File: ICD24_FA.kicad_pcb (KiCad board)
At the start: 2 copper layers, 201.5 x 218 mm, 446 parts, among them J1 Conn_01x02, Q342 2N3904, Q343 2N3904, Q344 2N3904, Q345 2N3904, Q346 2N3904, Q347 2N3904, Q348 2N3904, Q349 2N3904, Q350 2N3904, Q351 2N3904, Q352 2N3904, Q353 2N3904, Q354 2N3904, Q355 2N3904, Q356 2N3904, Q357 2N3904, Q358 2N3904, Q359 2N3904, Q360 2N3904, Q361 2N3904, Q362 2N3904, Q363 2N3904, Q364 2N3904, Q365 2N3904, Q366 2N3904, Q367 2N3904, Q368 2N3904, Q369 2N3904, Q370 2N3904, Q371 2N3904, Q372 2N3904, Q373 2N3904, Q374 2N3904, Q375 2N3904, Q376 2N3904, Q377 2N3904, Q378 2N3904, Q379 2N3904, Q380 2N3904, Q381 2N3904, Q382 2N3904, Q383 2N3904, Q384 2N3904, Q385 2N3904, Q386 2N3904, Q387 2N3904, Q388 2N3904, Q389 2N3904, Q390 2N3904, Q391 2N3904, Q392 2N3904, Q393 2N3904, Q394 2N3904, Q395 2N3904, Q396 2N3904, Q397 2N3904, Q398 2N3904, Q399 2N3904, Q400 2N3904, Q401 2N3904, Q402 2N3904, Q403 2N3904, Q404 2N3904, Q405 2N3904, Q406 2N3904, Q407 2N3904, Q408 2N3904, Q409 2N3904, Q410 2N3904, Q411 2N3904, Q412 2N3904, Q413 2N3904, Q414 2N3904, Q415 2N3904, Q416 2N3904, Q417 2N3904, Q418 2N3904, Q419 2N3904, Q420 2N3904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

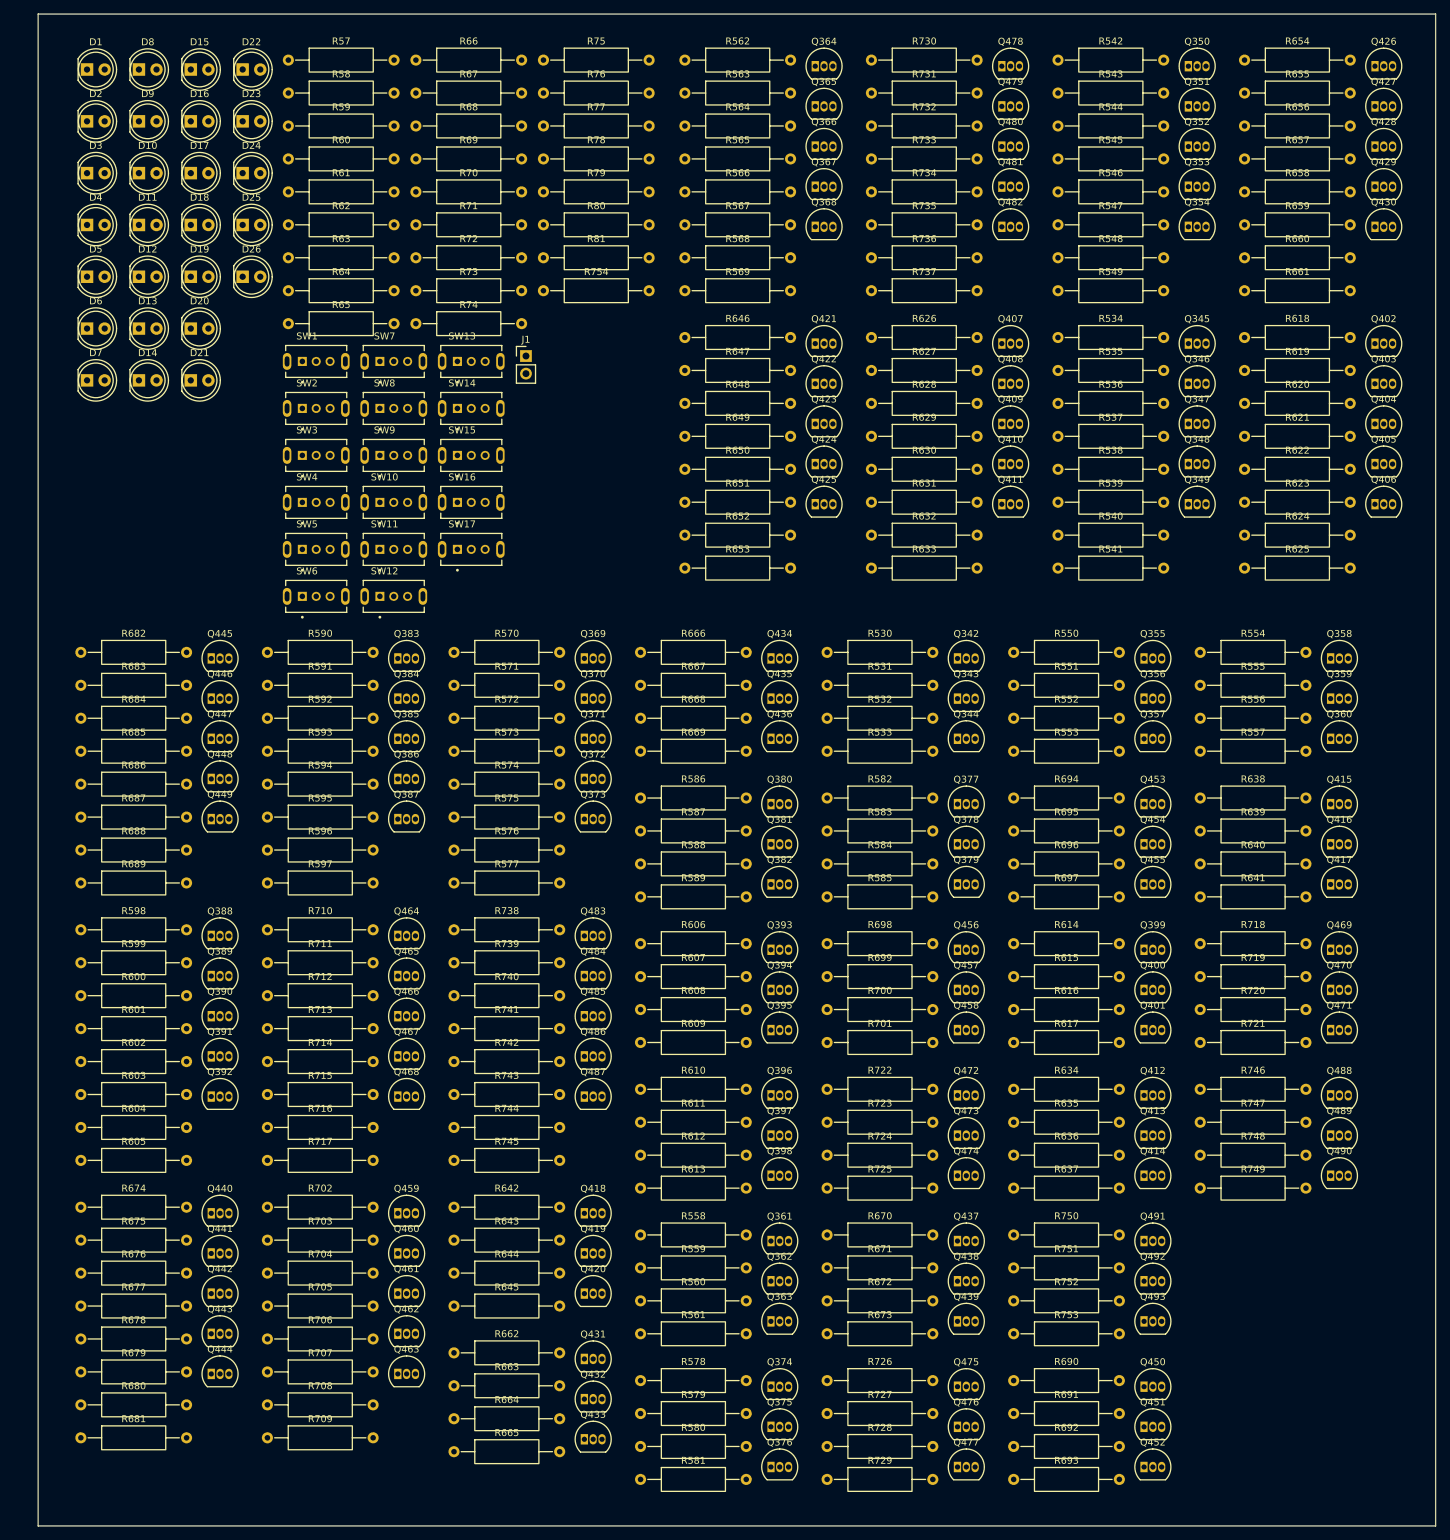
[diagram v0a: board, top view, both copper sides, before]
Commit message: FA 2-bit
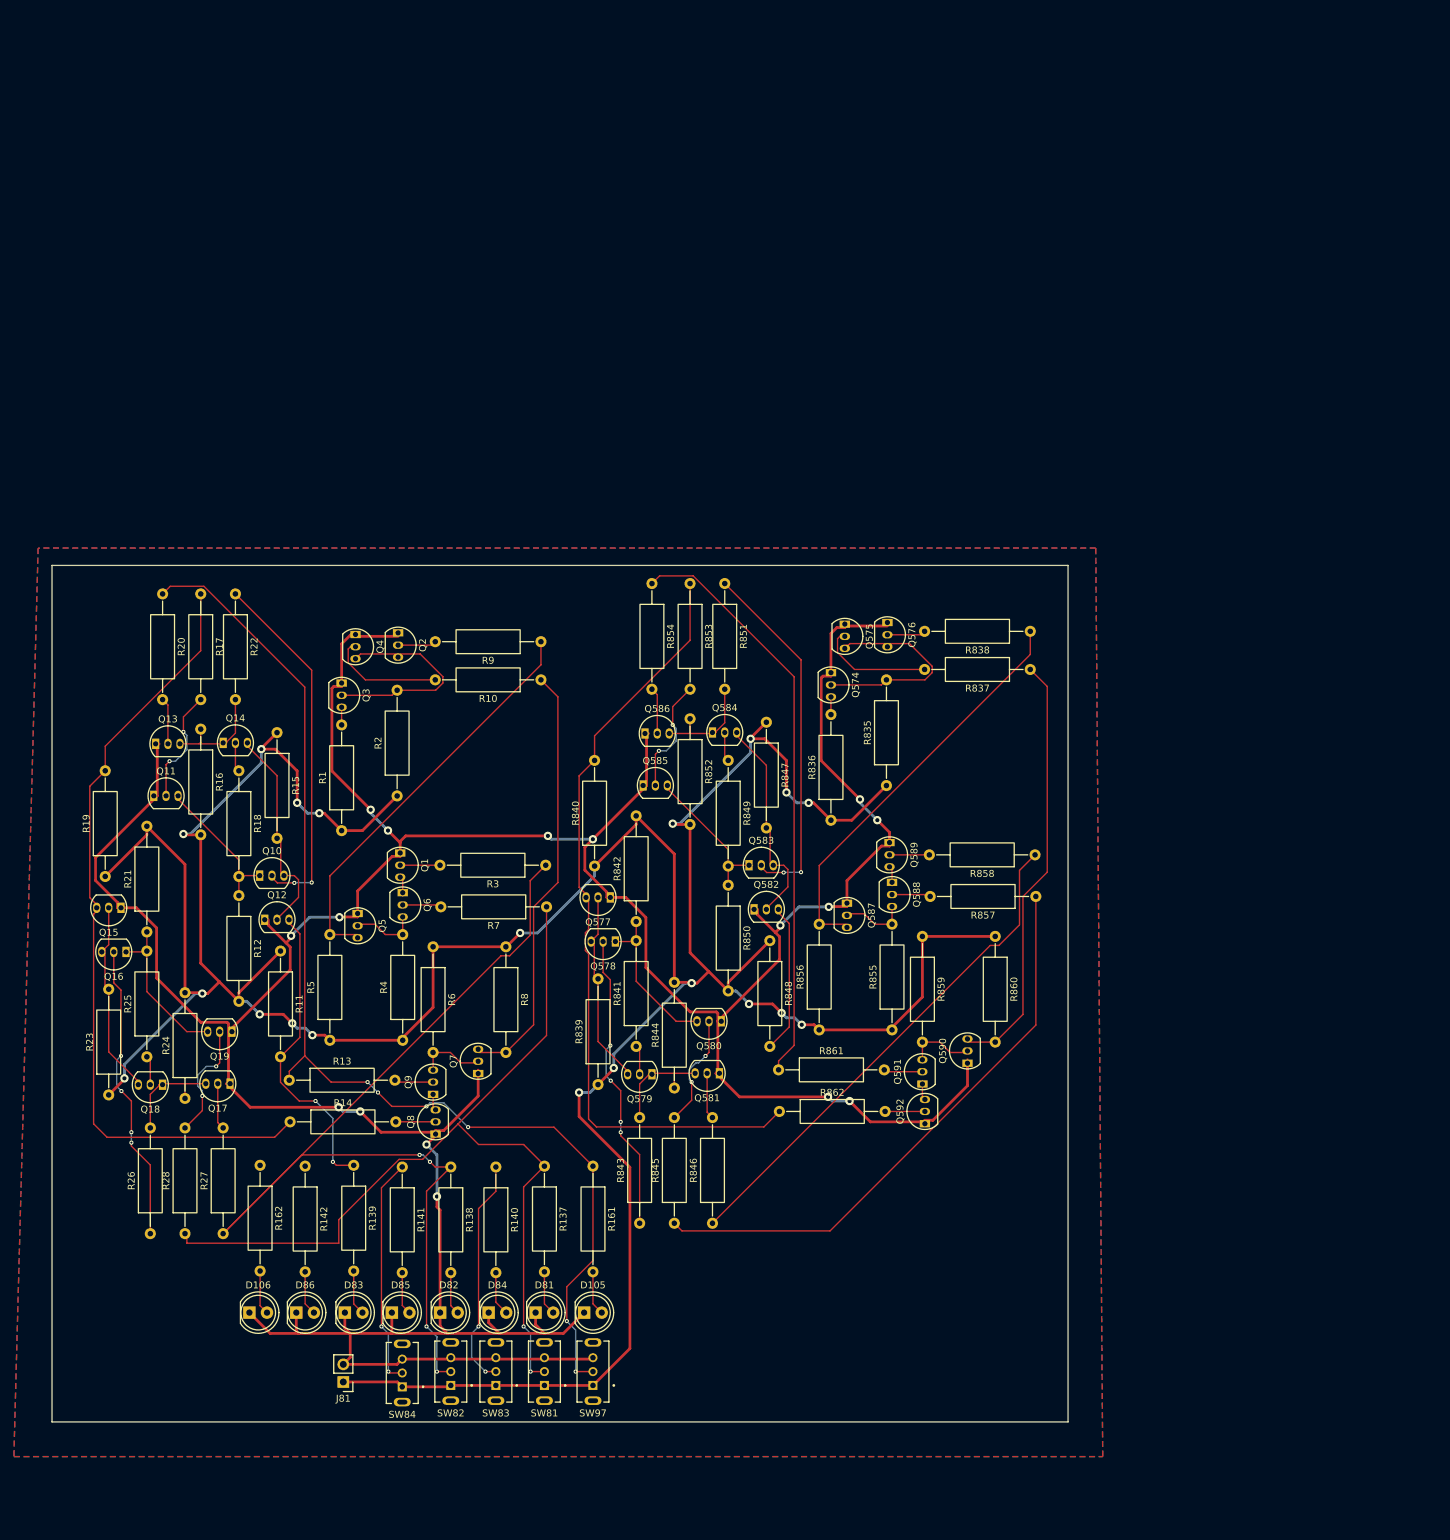
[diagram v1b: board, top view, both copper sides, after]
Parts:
- removed D1, D10, D11, D12, D13, D14, D15, D16, D17, D18, D19, D2, D20, D21, D22, D23, D24, D25, D26, D3, D4, D5, D6, D7, D8, D9: LED, LED_THT:LED_D5.0mm
- removed J1: Conn_01x02, Connector_PinHeader_2.54mm:PinHeader_1x02_P2.54mm_Vertical
- removed Q342, Q343, Q344, Q345, Q346, Q347, Q348, Q349, Q350, Q351, Q352, Q353, Q354, Q355, Q356, Q357, Q358, Q359, Q360, Q361, Q362, Q363, Q364, Q365, Q366, Q367, Q368, Q369, Q370, Q371, Q372, Q373, Q374, Q375, Q376, Q377, Q378, Q379, Q380, Q381, Q382, Q383, Q384, Q385, Q386, Q387, Q388, Q389, Q390, Q391, Q392, Q393, Q394, Q395, Q396, Q397, Q398, Q399, Q400, Q401, Q402, Q403, Q404, Q405, Q406, Q407, Q408, Q409, Q410, Q411, Q412, Q413, Q414, Q415, Q416, Q417, Q418, Q419, Q420, Q421, Q422, Q423, Q424, Q425, Q426, Q427, Q428, Q429, Q430, Q431, Q432, Q433, Q434, Q435, Q436, Q437, Q438, Q439, Q440, Q441, Q442, Q443, Q444, Q445, Q446, Q447, Q448, Q449, Q450, Q451, Q452, Q453, Q454, Q455, Q456, Q457, Q458, Q459, Q460, Q461, Q462, Q463, Q464, Q465, Q466, Q467, Q468, Q469, Q470, Q471, Q472, Q473, Q474, Q475, Q476, Q477, Q478, Q479, Q480, Q481, Q482, Q483, Q484, Q485, Q486, Q487, Q488, Q489, Q490, Q491, Q492, Q493: 2N3904, Package_TO_SOT_THT:TO-92_Inline
- removed R530, R531, R532, R534, R535, R536, R537, R538, R539, R540, R542, R543, R544, R545, R546, R547, R548, R550, R551, R552, R554, R555, R556, R558, R559, R560, R562, R563, R564, R565, R566, R567, R568, R570, R571, R572, R573, R574, R575, R576, R578, R579, R580, R582, R583, R584, R586, R587, R588, R590, R591, R592, R593, R594, R595, R596, R598, R599, R600, R601, R602, R603, R604, R606, R607, R608, R610, R611, R612, R614, R615, R616, R618, R619, R620, R621, R622, R623, R624, R626, R627, R628, R629, R630, R631, R632, R634, R635, R636, R638, R639, R640, R642, R643, R644, R646, R647, R648, R649, R650, R651, R652, R654, R655, R656, R657, R658, R659, R660, R662, R663, R664, R666, R667, R668, R670, R671, R672, R674, R675, R676, R677, R678, R679, R680, R682, R683, R684, R685, R686, R687, R688, R690, R691, R692, R694, R695, R696, R698, R699, R700, R702, R703, R704, R705, R706, R707, R708, R710, R711, R712, R713, R714, R715, R716, R718, R719, R720, R722, R723, R724, R726, R727, R728, R730, R731, R732, R733, R734, R735, R736, R738, R739, R740, R741, R742, R743, R744, R746, R747, R748, R750, R751, R752: 220k, Resistor_THT:R_Axial_DIN0309_L9.0mm_D3.2mm_P15.24mm_Horizontal
- removed R533, R541, R549, R553, R557, R561, R569, R57, R577, R58, R581, R585, R589, R59, R597, R60, R605, R609, R61, R613, R617, R62, R625, R63, R633, R637, R64, R641, R645, R65, R653, R66, R661, R665, R669, R67, R673, R68, R681, R689, R69, R693, R697, R70, R701, R709, R71, R717, R72, R721, R725, R729, R73, R737, R74, R745, R749, R75, R753, R754, R76, R77, R78, R79, R80, R81: 47k, Resistor_THT:R_Axial_DIN0309_L9.0mm_D3.2mm_P15.24mm_Horizontal
- removed SW1, SW10, SW11, SW12, SW13, SW14, SW15, SW16, SW17, SW2, SW3, SW4, SW5, SW6, SW7, SW8, SW9: SW_SPDT, MyLibrary:SW_SS12D07VG4
- added D105: LED, LED_THT:LED_D5.0mm, F.Cu at (170.7, 220.2)
- added D106: LED, LED_THT:LED_D5.0mm, F.Cu at (122.5, 220.2)
- added D81: LED, LED_THT:LED_D5.0mm, F.Cu at (163.7, 220.2)
- added D82: LED, LED_THT:LED_D5.0mm, F.Cu at (150.0, 220.2)
- added D83: LED, LED_THT:LED_D5.0mm, F.Cu at (136.2, 220.2)
- added D84: LED, LED_THT:LED_D5.0mm, F.Cu at (157.0, 220.2)
- added D85: LED, LED_THT:LED_D5.0mm, F.Cu at (143.0, 220.2)
- added D86: LED, LED_THT:LED_D5.0mm, F.Cu at (129.2, 220.2)
- added J81: Conn_01x02, Connector_PinHeader_2.54mm:PinHeader_1x02_P2.54mm_Vertical, F.Cu at (136.0, 230.2)
- added Q1: 2N3904, MyLibrary:TO-92_Inline, F.Cu at (144.2, 154.5)
- added Q10: 2N3904, MyLibrary:TO-92_Inline, F.Cu at (124.4, 157.2)
- added Q11: 2N3904, MyLibrary:TO-92_Inline, F.Cu at (109.2, 145.7)
- added Q12: 2N3904, MyLibrary:TO-92_Inline, F.Cu at (125.2, 163.6)
- added Q13: 2N3904, MyLibrary:TO-92_Inline, F.Cu at (109.4, 138.2)
- added Q14: 2N3904, MyLibrary:TO-92_Inline, F.Cu at (119.2, 138.1)
- added Q15: 2N3904, MyLibrary:TO-92_Inline, F.Cu at (103.4, 161.9)
- added Q16: 2N3904, MyLibrary:TO-92_Inline, F.Cu at (104.2, 168.2)
- added Q17: 2N3904, MyLibrary:TO-92_Inline, F.Cu at (119.2, 187.2)
- added Q18: 2N3904, MyLibrary:TO-92_Inline, F.Cu at (109.4, 187.4)
- added Q19: 2N3904, MyLibrary:TO-92_Inline, F.Cu at (119.4, 179.7)
- added Q2: 2N3904, MyLibrary:TO-92_Inline, F.Cu at (143.9, 122.7)
- added Q3: 2N3904, MyLibrary:TO-92_Inline, F.Cu at (135.8, 130.0)
- added Q4: 2N3904, MyLibrary:TO-92_Inline, F.Cu at (137.8, 123.0)
- added Q5: 2N3904, MyLibrary:TO-92_Inline, F.Cu at (138.1, 163.2)
- added Q574: 2N3904, MyLibrary:TO-92_Inline, F.Cu at (206.3, 128.5)
- added Q575: 2N3904, MyLibrary:TO-92_Inline, F.Cu at (208.3, 121.5)
- added Q576: 2N3904, MyLibrary:TO-92_Inline, F.Cu at (214.5, 121.2)
- added Q577: 2N3904, MyLibrary:TO-92_Inline, F.Cu at (174.0, 160.4)
- added Q578: 2N3904, MyLibrary:TO-92_Inline, F.Cu at (174.7, 166.7)
- added Q579: 2N3904, MyLibrary:TO-92_Inline, F.Cu at (180.0, 185.9)
- added Q580: 2N3904, MyLibrary:TO-92_Inline, F.Cu at (190.0, 178.2)
- added Q581: 2N3904, MyLibrary:TO-92_Inline, F.Cu at (189.7, 185.7)
- added Q582: 2N3904, MyLibrary:TO-92_Inline, F.Cu at (195.7, 162.1)
- added Q583: 2N3904, MyLibrary:TO-92_Inline, F.Cu at (195.0, 155.7)
- added Q584: 2N3904, MyLibrary:TO-92_Inline, F.Cu at (189.7, 136.6)
- added Q585: 2N3904, MyLibrary:TO-92_Inline, F.Cu at (179.7, 144.2)
- added Q586: 2N3904, MyLibrary:TO-92_Inline, F.Cu at (180.0, 136.7)
- added Q587: 2N3904, MyLibrary:TO-92_Inline, F.Cu at (208.6, 161.7)
- added Q588: 2N3904, MyLibrary:TO-92_Inline, F.Cu at (215.1, 158.7)
- added Q589: 2N3904, MyLibrary:TO-92_Inline, F.Cu at (214.8, 153.0)
- added Q590: 2N3904, MyLibrary:TO-92_Inline, F.Cu at (226.0, 183.8)
- added Q591: 2N3904, MyLibrary:TO-92_Inline, F.Cu at (219.5, 186.8)
- added Q592: 2N3904, MyLibrary:TO-92_Inline, F.Cu at (219.9, 192.5)
- added Q6: 2N3904, MyLibrary:TO-92_Inline, F.Cu at (144.6, 160.2)
- added Q7: 2N3904, MyLibrary:TO-92_Inline, F.Cu at (155.4, 185.3)
- added Q8: 2N3904, MyLibrary:TO-92_Inline, F.Cu at (149.3, 194.0)
- added Q9: 2N3904, MyLibrary:TO-92_Inline, F.Cu at (148.9, 188.3)
- added R1: 47k, Resistor_THT:R_Axial_DIN0309_L9.0mm_D3.2mm_P15.24mm_Horizontal, F.Cu at (135.8, 150.7)
- added R10: 220k, Resistor_THT:R_Axial_DIN0309_L9.0mm_D3.2mm_P15.24mm_Horizontal, F.Cu at (164.5, 129.0)
- added R11: 47k, Resistor_THT:R_Axial_DIN0309_L9.0mm_D3.2mm_P15.24mm_Horizontal, F.Cu at (126.9, 168.1)
- added R12: 220k, Resistor_THT:R_Axial_DIN0309_L9.0mm_D3.2mm_P15.24mm_Horizontal, F.Cu at (120.9, 160.1)
- added R13: 220k, Resistor_THT:R_Axial_DIN0309_L9.0mm_D3.2mm_P15.24mm_Horizontal, F.Cu at (128.2, 186.7)
- added R137: 47k, Resistor_THT:R_Axial_DIN0309_L9.0mm_D3.2mm_P15.24mm_Horizontal, F.Cu at (165.0, 199.1)
- added R138: 47k, Resistor_THT:R_Axial_DIN0309_L9.0mm_D3.2mm_P15.24mm_Horizontal, F.Cu at (151.5, 199.2)
- added R139: 47k, Resistor_THT:R_Axial_DIN0309_L9.0mm_D3.2mm_P15.24mm_Horizontal, F.Cu at (137.5, 199.0)
- added R14: 220k, Resistor_THT:R_Axial_DIN0309_L9.0mm_D3.2mm_P15.24mm_Horizontal, F.Cu at (128.3, 192.7)
- added R140: 47k, Resistor_THT:R_Axial_DIN0309_L9.0mm_D3.2mm_P15.24mm_Horizontal, F.Cu at (158.0, 199.2)
- added R141: 47k, Resistor_THT:R_Axial_DIN0309_L9.0mm_D3.2mm_P15.24mm_Horizontal, F.Cu at (144.5, 199.2)
- added R142: 47k, Resistor_THT:R_Axial_DIN0309_L9.0mm_D3.2mm_P15.24mm_Horizontal, F.Cu at (130.5, 199.1)
- added R15: 220k, Resistor_THT:R_Axial_DIN0309_L9.0mm_D3.2mm_P15.24mm_Horizontal, F.Cu at (126.4, 136.6)
- added R16: 220k, Resistor_THT:R_Axial_DIN0309_L9.0mm_D3.2mm_P15.24mm_Horizontal, F.Cu at (115.4, 136.1)
- added R161: 47k, Resistor_THT:R_Axial_DIN0309_L9.0mm_D3.2mm_P15.24mm_Horizontal, F.Cu at (172.0, 199.1)
- added R162: 47k, Resistor_THT:R_Axial_DIN0309_L9.0mm_D3.2mm_P15.24mm_Horizontal, F.Cu at (124.0, 199.0)
- added R17: 220k, Resistor_THT:R_Axial_DIN0309_L9.0mm_D3.2mm_P15.24mm_Horizontal, F.Cu at (115.4, 116.6)
- added R18: 220k, Resistor_THT:R_Axial_DIN0309_L9.0mm_D3.2mm_P15.24mm_Horizontal, F.Cu at (120.9, 142.1)
- added R19: 47k, Resistor_THT:R_Axial_DIN0309_L9.0mm_D3.2mm_P15.24mm_Horizontal, F.Cu at (101.7, 157.3)
- added R2: 220k, Resistor_THT:R_Axial_DIN0309_L9.0mm_D3.2mm_P15.24mm_Horizontal, F.Cu at (143.8, 145.7)
- added R20: 220k, Resistor_THT:R_Axial_DIN0309_L9.0mm_D3.2mm_P15.24mm_Horizontal, F.Cu at (109.9, 116.6)
- added R21: 220k, Resistor_THT:R_Axial_DIN0309_L9.0mm_D3.2mm_P15.24mm_Horizontal, F.Cu at (107.7, 165.3)
- added R22: 220k, Resistor_THT:R_Axial_DIN0309_L9.0mm_D3.2mm_P15.24mm_Horizontal, F.Cu at (120.4, 116.6)
- added R23: 220k, Resistor_THT:R_Axial_DIN0309_L9.0mm_D3.2mm_P15.24mm_Horizontal, F.Cu at (102.2, 188.8)
- added R24: 220k, Resistor_THT:R_Axial_DIN0309_L9.0mm_D3.2mm_P15.24mm_Horizontal, F.Cu at (113.2, 189.3)
- added R25: 220k, Resistor_THT:R_Axial_DIN0309_L9.0mm_D3.2mm_P15.24mm_Horizontal, F.Cu at (107.7, 183.3)
- added R26: 220k, Resistor_THT:R_Axial_DIN0309_L9.0mm_D3.2mm_P15.24mm_Horizontal, F.Cu at (108.2, 208.8)
- added R27: 220k, Resistor_THT:R_Axial_DIN0309_L9.0mm_D3.2mm_P15.24mm_Horizontal, F.Cu at (118.7, 208.8)
- added R28: 220k, Resistor_THT:R_Axial_DIN0309_L9.0mm_D3.2mm_P15.24mm_Horizontal, F.Cu at (113.2, 208.8)
- added R3: 220k, Resistor_THT:R_Axial_DIN0309_L9.0mm_D3.2mm_P15.24mm_Horizontal, F.Cu at (165.2, 155.7)
- added R4: 220k, Resistor_THT:R_Axial_DIN0309_L9.0mm_D3.2mm_P15.24mm_Horizontal, F.Cu at (144.6, 181.0)
- added R5: 47k, Resistor_THT:R_Axial_DIN0309_L9.0mm_D3.2mm_P15.24mm_Horizontal, F.Cu at (134.1, 181.0)
- added R6: 220k, Resistor_THT:R_Axial_DIN0309_L9.0mm_D3.2mm_P15.24mm_Horizontal, F.Cu at (148.9, 167.5)
- added R7: 220k, Resistor_THT:R_Axial_DIN0309_L9.0mm_D3.2mm_P15.24mm_Horizontal, F.Cu at (165.3, 161.7)
- added R8: 47k, Resistor_THT:R_Axial_DIN0309_L9.0mm_D3.2mm_P15.24mm_Horizontal, F.Cu at (159.4, 167.5)
- added R835: 220k, Resistor_THT:R_Axial_DIN0309_L9.0mm_D3.2mm_P15.24mm_Horizontal, F.Cu at (214.3, 144.2)
- added R836: 47k, Resistor_THT:R_Axial_DIN0309_L9.0mm_D3.2mm_P15.24mm_Horizontal, F.Cu at (206.3, 149.2)
- added R837: 220k, Resistor_THT:R_Axial_DIN0309_L9.0mm_D3.2mm_P15.24mm_Horizontal, F.Cu at (235.1, 127.5)
- added R838: 220k, Resistor_THT:R_Axial_DIN0309_L9.0mm_D3.2mm_P15.24mm_Horizontal, F.Cu at (235.1, 122.0)
- added R839: 220k, Resistor_THT:R_Axial_DIN0309_L9.0mm_D3.2mm_P15.24mm_Horizontal, F.Cu at (172.7, 187.4)
- added R840: 47k, Resistor_THT:R_Axial_DIN0309_L9.0mm_D3.2mm_P15.24mm_Horizontal, F.Cu at (172.2, 155.9)
- added R841: 220k, Resistor_THT:R_Axial_DIN0309_L9.0mm_D3.2mm_P15.24mm_Horizontal, F.Cu at (178.2, 181.9)
- added R842: 220k, Resistor_THT:R_Axial_DIN0309_L9.0mm_D3.2mm_P15.24mm_Horizontal, F.Cu at (178.2, 163.9)
- added R843: 220k, Resistor_THT:R_Axial_DIN0309_L9.0mm_D3.2mm_P15.24mm_Horizontal, F.Cu at (178.7, 207.4)
- added R844: 220k, Resistor_THT:R_Axial_DIN0309_L9.0mm_D3.2mm_P15.24mm_Horizontal, F.Cu at (183.7, 187.9)
- added R845: 220k, Resistor_THT:R_Axial_DIN0309_L9.0mm_D3.2mm_P15.24mm_Horizontal, F.Cu at (183.7, 207.4)
- added R846: 220k, Resistor_THT:R_Axial_DIN0309_L9.0mm_D3.2mm_P15.24mm_Horizontal, F.Cu at (189.2, 207.4)
- added R847: 220k, Resistor_THT:R_Axial_DIN0309_L9.0mm_D3.2mm_P15.24mm_Horizontal, F.Cu at (197.0, 135.1)
- added R848: 47k, Resistor_THT:R_Axial_DIN0309_L9.0mm_D3.2mm_P15.24mm_Horizontal, F.Cu at (197.5, 166.6)
- added R849: 220k, Resistor_THT:R_Axial_DIN0309_L9.0mm_D3.2mm_P15.24mm_Horizontal, F.Cu at (191.5, 140.6)
- added R850: 220k, Resistor_THT:R_Axial_DIN0309_L9.0mm_D3.2mm_P15.24mm_Horizontal, F.Cu at (191.5, 158.6)
- added R851: 220k, Resistor_THT:R_Axial_DIN0309_L9.0mm_D3.2mm_P15.24mm_Horizontal, F.Cu at (191.0, 115.1)
- added R852: 220k, Resistor_THT:R_Axial_DIN0309_L9.0mm_D3.2mm_P15.24mm_Horizontal, F.Cu at (186.0, 134.6)
- added R853: 220k, Resistor_THT:R_Axial_DIN0309_L9.0mm_D3.2mm_P15.24mm_Horizontal, F.Cu at (186.0, 115.1)
- added R854: 220k, Resistor_THT:R_Axial_DIN0309_L9.0mm_D3.2mm_P15.24mm_Horizontal, F.Cu at (180.5, 115.1)
- added R855: 220k, Resistor_THT:R_Axial_DIN0309_L9.0mm_D3.2mm_P15.24mm_Horizontal, F.Cu at (215.1, 179.5)
- added R856: 47k, Resistor_THT:R_Axial_DIN0309_L9.0mm_D3.2mm_P15.24mm_Horizontal, F.Cu at (204.6, 179.5)
- added R857: 220k, Resistor_THT:R_Axial_DIN0309_L9.0mm_D3.2mm_P15.24mm_Horizontal, F.Cu at (235.9, 160.2)
- added R858: 220k, Resistor_THT:R_Axial_DIN0309_L9.0mm_D3.2mm_P15.24mm_Horizontal, F.Cu at (235.7, 154.2)
- added R859: 220k, Resistor_THT:R_Axial_DIN0309_L9.0mm_D3.2mm_P15.24mm_Horizontal, F.Cu at (219.5, 166.0)
- added R860: 47k, Resistor_THT:R_Axial_DIN0309_L9.0mm_D3.2mm_P15.24mm_Horizontal, F.Cu at (230.0, 166.0)
- added R861: 220k, Resistor_THT:R_Axial_DIN0309_L9.0mm_D3.2mm_P15.24mm_Horizontal, F.Cu at (198.8, 185.2)
- added R862: 220k, Resistor_THT:R_Axial_DIN0309_L9.0mm_D3.2mm_P15.24mm_Horizontal, F.Cu at (198.9, 191.2)
- added R9: 220k, Resistor_THT:R_Axial_DIN0309_L9.0mm_D3.2mm_P15.24mm_Horizontal, F.Cu at (164.5, 123.5)
- added SW81: SW_SPDT, MyLibrary:SW_SS12D07VG4, F.Cu at (165.0, 228.7)
- added SW82: SW_SPDT, MyLibrary:SW_SS12D07VG4, F.Cu at (151.5, 228.7)
- added SW83: SW_SPDT, MyLibrary:SW_SS12D07VG4, F.Cu at (158.0, 228.7)
- added SW84: SW_SPDT, MyLibrary:SW_SS12D07VG4, F.Cu at (144.5, 228.9)
- added SW97: SW_SPDT, MyLibrary:SW_SS12D07VG4, F.Cu at (172.0, 228.7)
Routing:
- net 0: track 0.00 -> 567.2 mm, vias 0 -> 16
- net VDD: track 0.00 -> 511.1 mm, vias 0 -> 20
- net CIN: track 0.00 -> 167.4 mm, vias 0 -> 6
- net IN_B0: track 0.00 -> 144.9 mm, vias 0 -> 4
- net IN_A0: track 0.00 -> 134.6 mm, vias 0 -> 2
- net /fa2_bit/fa1/and_gate/IN_B: track 0.00 -> 114.1 mm
- net /fa2_bit/fa2/and_gate/IN_B: track 0.00 -> 113.8 mm
- net /fa2_bit/fa2/CIN: track 0.00 -> 84.6 mm
- net /fa2_bit/fa2/A: track 0.00 -> 83.4 mm
- net /fa2_bit/fa2/B: track 0.00 -> 73.1 mm
- net /fa2_bit/fa2/and_gate/OUT: track 0.00 -> 61.8 mm
- net /fa2_bit/fa1/and_gate/OUT: track 0.00 -> 61.8 mm
- net /fa2_bit/fa2/and_gate1/OUT: track 0.00 -> 58.8 mm
- net /fa2_bit/fa1/and_gate1/OUT: track 0.00 -> 58.8 mm
- net Net-(Q10-B): track 0.00 -> 52.5 mm, vias 0 -> 2
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- added copper zone on B.Cu, net 0
- added copper zone on F.Cu, net 0
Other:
- board size 201.5 x 218 mm -> 146.5 x 123.5 mm
